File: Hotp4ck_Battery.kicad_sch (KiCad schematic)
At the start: 16 parts, among them J3 Conn_01x02_MountingPin, Q1 AO3401A, SW2 PWR, U3 MAX17048, U3 TP4056

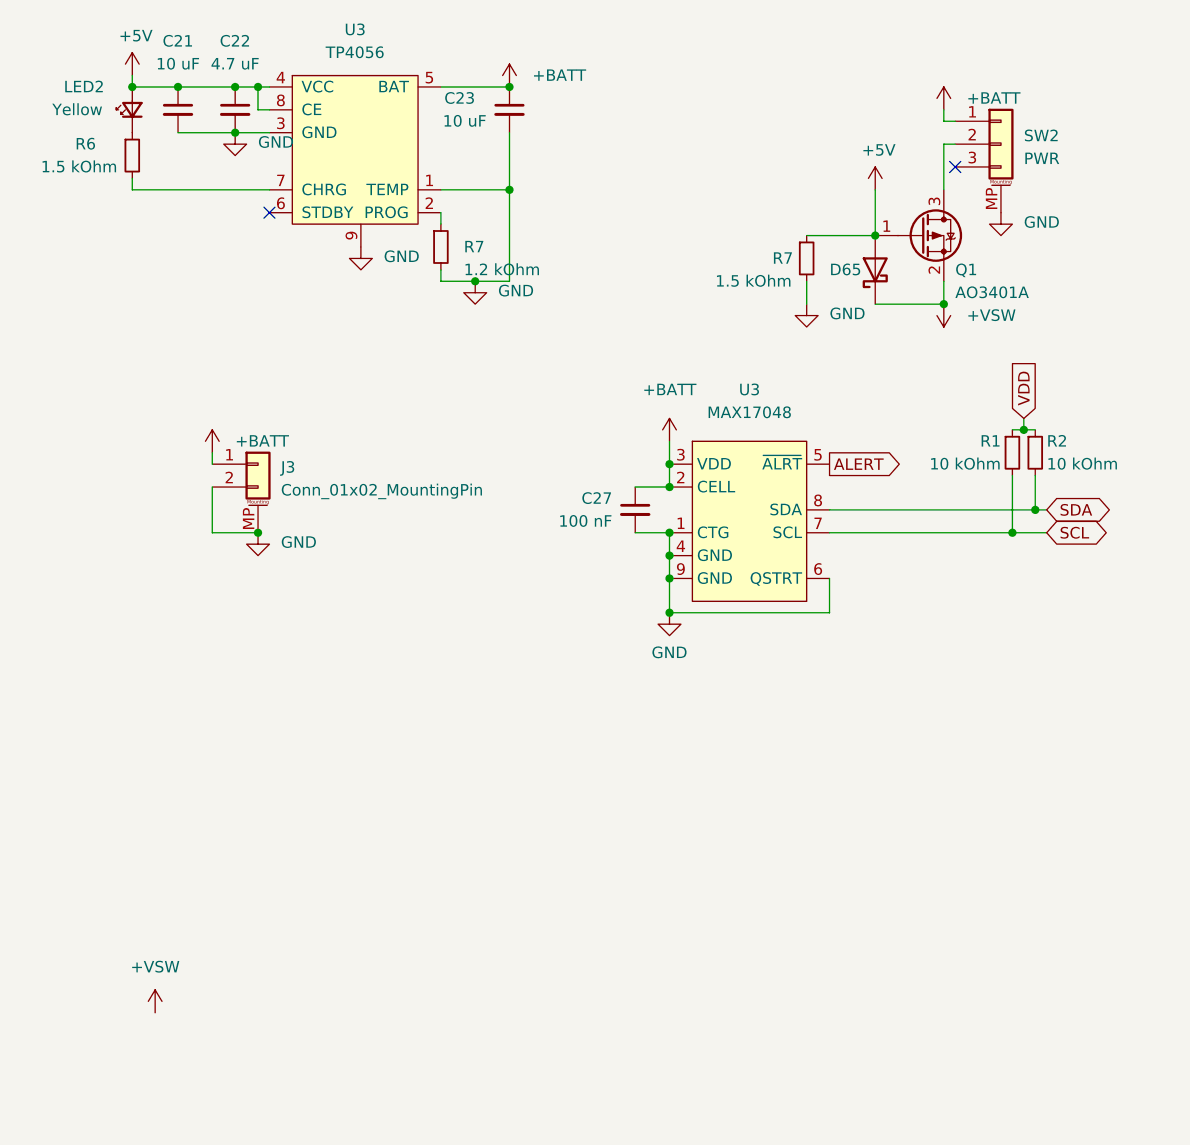
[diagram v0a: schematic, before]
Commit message: Make Readme.md
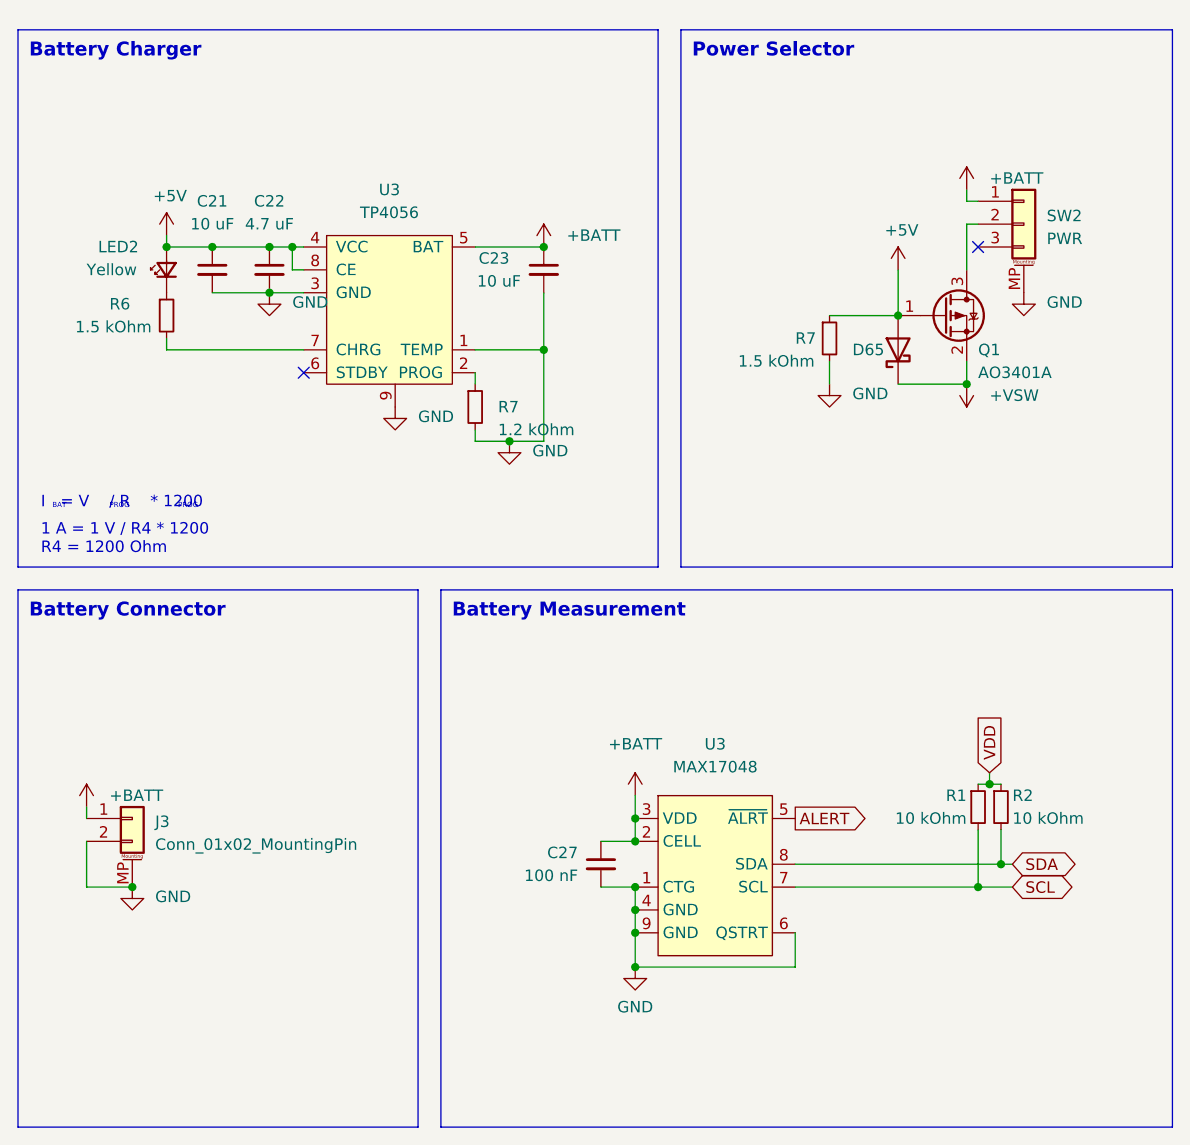
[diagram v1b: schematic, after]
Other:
- note added: "1 A = 1 V / R4 * 1200 R4 = 1200 Ohm"
- note added: "BAT"
- note added: "I = V / R * 1200"
- note added: "PROG"
- moved on the sheet: C21, C22, C23, C27, D65, J3, LED2, Q1, R1, R2, R6, R7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
